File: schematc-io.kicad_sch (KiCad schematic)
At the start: 36 parts, among them IC1 AD8544ARUZ-REEL, U3 SN65HVD232

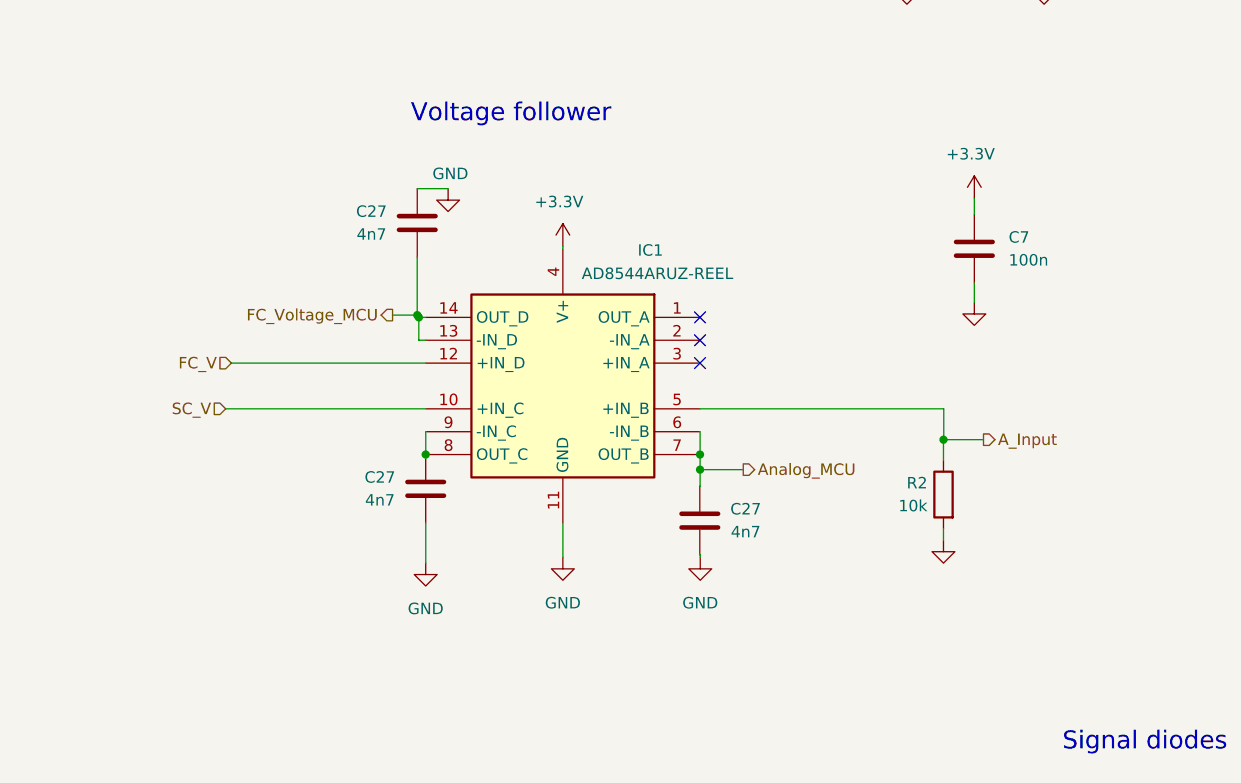
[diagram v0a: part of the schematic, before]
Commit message: Edit mosfets outputs
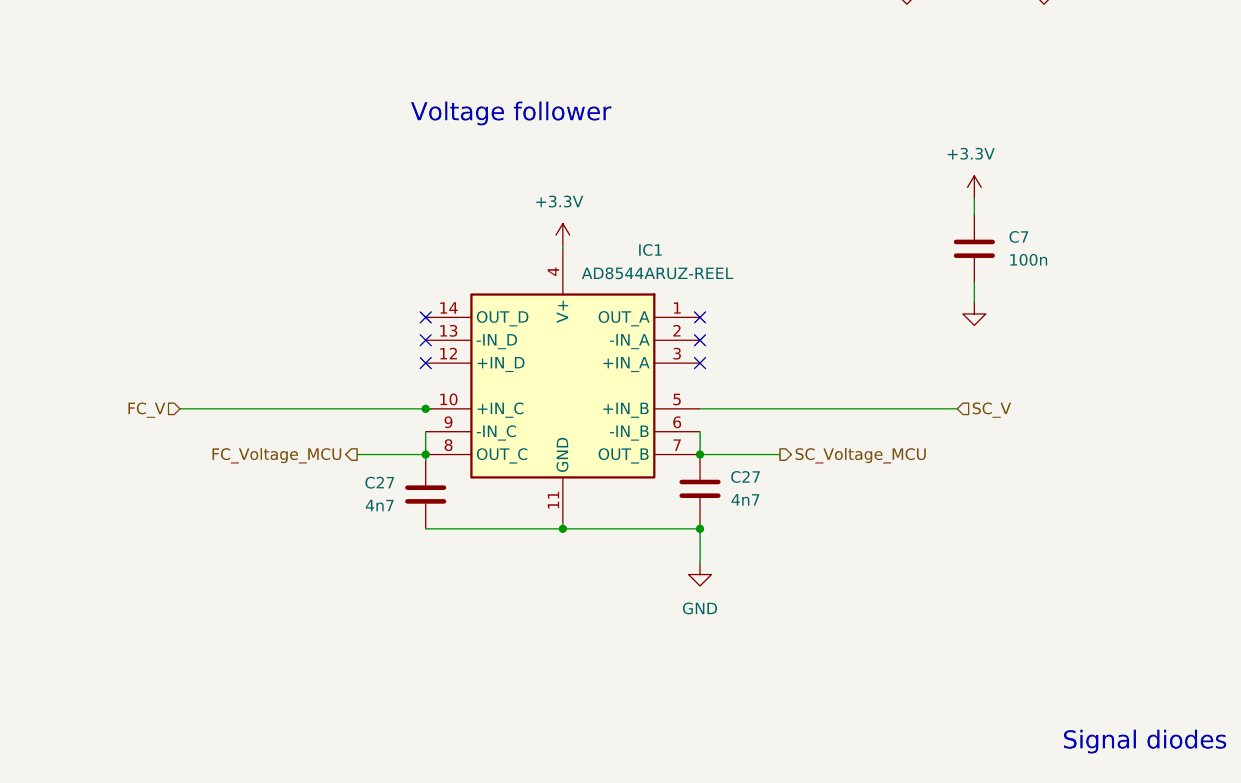
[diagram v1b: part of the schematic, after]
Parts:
- removed C27 (x3): 4n7, Capacitor_SMD:C_1206_3216Metric, symbol Device:C
- removed R2: 10k, LED_SMD:LED_1206_3216Metric, symbol Device:R
- added C27 (x2): 4n7, Capacitor_SMD:C_1206_3216Metric, symbol Device:C
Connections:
- net A_Input is gone; now on net SC_V: IC1.5 (+IN_B)
- net FC_V: now also IC1.10 (+IN_C); no longer IC1.12 (+IN_D)
- net FC_Voltage_MCU: now also IC1.8 (OUT_C), IC1.9 (-IN_C), C27.1; no longer IC1.13 (-IN_D), IC1.14 (OUT_D)
- net GND: now also C27.2, C27.2
- net SC_V: no longer IC1.10 (+IN_C)
- net Analog_MCU renamed SC_Voltage_MCU
- net SC_Voltage_MCU: now also C27.1
- no-connect marks 3 -> 6
